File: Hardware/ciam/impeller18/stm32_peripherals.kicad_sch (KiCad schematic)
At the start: 31 parts, among them J21 TF-01, J22 USB_B_Micro, U73 W25Q128FVSIG, U74 USBLC6-2SC6

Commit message: added footprints
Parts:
- C108, C109, C110: footprint (none) -> Capacitor_SMD:C_0603_1608Metric
- D21, D22, D23, D24: footprint (none) -> user_lib:LED_RGB_promelec
- J22: footprint (none) -> user_lib:U-F-M5DD-W-2-SUS
- R259, R260, R261, R262, R263, R264, R265, R266, R267, R268, R269, R270, R271, R272, R273, R274, R275, R276, R277, R278: footprint (none) -> Resistor_SMD:R_0603_1608Metric
- U73: footprint (none) -> Package_SO:SOIC-8_5.23x5.23mm_P1.27mm
- U74: footprint (none) -> Package_TO_SOT_SMD:SOT-23-6
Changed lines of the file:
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@@
 			)
 		)
-		(property "Footprint" ""
+		(property "Footprint" "Resistor_SMD:R_0603_1608Metric"
 			(at 249.555 40.513 90)
 			(effects
@@
 			)
 		)
-		(property "Footprint" ""
+		(property "Footprint" "Resistor_SMD:R_0603_1608Metric"
 			(at 249.555 57.658 90)
 			(effects
@@
 			)
 		)
-		(property "Footprint" ""
+		(property "Footprint" "Resistor_SMD:R_0603_1608Metric"
 			(at 249.555 62.738 90)
 			(effects
@@
 			)
 		)
-		(property "Footprint" ""
+		(property "Footprint" "Resistor_SMD:R_0603_1608Metric"
 			(at 57.785 32.385 0)
 			(effects
@@
 			)
 		)
-		(property "Footprint" ""
+		(property "Footprint" "Resistor_SMD:R_0603_1608Metric"
 			(at 249.555 35.433 90)
 			(effects
@@
 			)
 		)
-		(property "Footprint" ""
+		(property "Footprint" "Resistor_SMD:R_0603_1608Metric"
 			(at 308.61 40.513 90)
 			(effects
@@
 			)
 		)
-		(property "Footprint" ""
+		(property "Footprint" "Resistor_SMD:R_0603_1608Metric"
 			(at 308.61 62.738 90)
 			(effects
@@
 			)
 		)
-		(property "Footprint" ""
+		(property "Footprint" "Package_SO:SOIC-8_5.23x5.23mm_P1.27mm"
 			(at 189.23 49.53 0)
 			(effects
@@
 			)
 		)
-		(property "Footprint" ""
+		(property "Footprint" "Resistor_SMD:R_0603_1608Metric"
 			(at 308.61 57.658 90)
 			(effects
@@
 			)
 		)
-		(property "Footprint" ""
+		(property "Footprint" "Resistor_SMD:R_0603_1608Metric"
 			(at 73.025 32.385 0)
 			(effects
@@
 			)
 		)
-		(property "Footprint" ""
+		(property "Footprint" "Capacitor_SMD:C_0603_1608Metric"
 			(at 30.48 114.935 0)
 			(effects
@@
 			)
 		)
-		(property "Footprint" ""
+		(property "Footprint" "Resistor_SMD:R_0603_1608Metric"
 			(at 120.015 119.38 0)
 			(effects
@@
 			)
 		)
-		(property "Footprint" ""
+		(property "Footprint" "Resistor_SMD:R_0603_1608Metric"
 			(at 50.165 32.385 0)
 			(effects
@@
 			)
 		)
-		(property "Footprint" ""
+		(property "Footprint" "Capacitor_SMD:C_0603_1608Metric"
 			(at 202.565 49.53 0)
 			(effects
@@
 			)
 		)
-		(property "Footprint" ""
+		(property "Footprint" "Package_TO_SOT_SMD:SOT-23-6"
 			(at 85.725 128.27 0)
 			(effects
@@
 			)
 		)
-		(property "Footprint" ""
+		(property "Footprint" "Resistor_SMD:R_0603_1608Metric"
 			(at 65.405 32.385 0)
 			(effects
@@
 			)
 		)
-		(property "Footprint" ""
+		(property "Footprint" "Resistor_SMD:R_0603_1608Metric"
 			(at 249.555 67.818 90)
 			(effects
@@
 			)
 		)
-		(property "Footprint" ""
+		(property "Footprint" "user_lib:U-F-M5DD-W-2-SUS"
 			(at 43.815 115.57 0)
 			(effects
@@
 			)
 		)
-		(property "Footprint" ""
+		(property "Footprint" "Resistor_SMD:R_0603_1608Metric"
 			(at 249.555 30.353 90)
 			(effects
@@
 			)
 		)
-		(property "Footprint" ""
+		(property "Footprint" "Resistor_SMD:R_0603_1608Metric"
 			(at 80.645 32.385 0)
 			(effects
@@
 			)
 		)
-		(property "Footprint" ""
+		(property "Footprint" "user_lib:LED_RGB_promelec"
 			(at 297.18 34.925 0)
 			(effects
@@
 			)
 		)
-		(property "Footprint" ""
+		(property "Footprint" "user_lib:LED_RGB_promelec"
 			(at 238.125 34.925 0)
 			(effects
@@
 			)
 		)
-		(property "Footprint" ""
+		(property "Footprint" "user_lib:LED_RGB_promelec"
 			(at 297.18 62.23 0)
 			(effects
@@
 			)
 		)
-		(property "Footprint" ""
+		(property "Footprint" "Resistor_SMD:R_0603_1608Metric"
 			(at 308.61 35.433 90)
 			(effects
@@
 			)
 		)
-		(property "Footprint" ""
+		(property "Footprint" "Resistor_SMD:R_0603_1608Metric"
 			(at 308.61 30.353 90)
 			(effects
@@
 			)
 		)
-		(property "Footprint" ""
+		(property "Footprint" "Resistor_SMD:R_0603_1608Metric"
 			(at 308.61 67.818 90)
 			(effects
@@
 			)
 		)
-		(property "Footprint" ""
+		(property "Footprint" "Resistor_SMD:R_0603_1608Metric"
 			(at 42.545 32.385 0)
 			(effects
@@
 			)
 		)
-		(property "Footprint" ""
+		(property "Footprint" "user_lib:LED_RGB_promelec"
 			(at 238.125 62.23 0)
 			(effects
@@
 			)
 		)
-		(property "Footprint" ""
+		(property "Footprint" "Capacitor_SMD:C_0603_1608Metric"
 			(at 97.79 28.575 0)
 			(effects
@@
 			)
 		)
-		(property "Footprint" ""
+		(property "Footprint" "Resistor_SMD:R_0603_1608Metric"
 			(at 120.015 109.22 0)
 			(effects

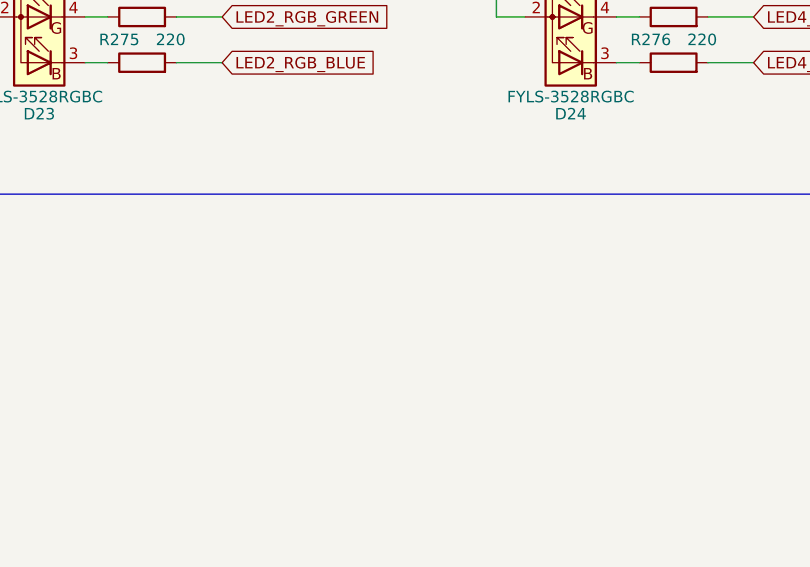
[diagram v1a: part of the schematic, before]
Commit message: Minor changes
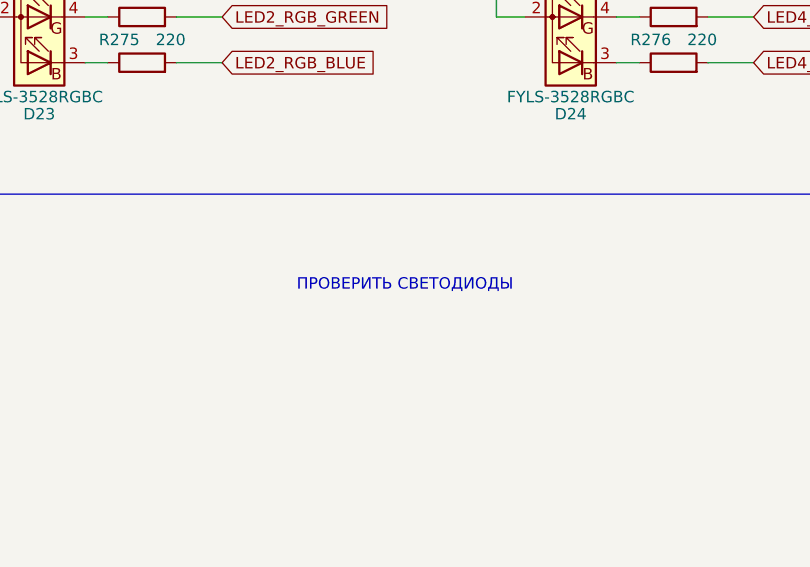
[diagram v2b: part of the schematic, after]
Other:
- note added: "ПРОВЕРИТЬ СВЕТОДИОДЫ"
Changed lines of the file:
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@@
+		)
+	)
+	(text "ПРОВЕРИТЬ СВЕТОДИОДЫ"
+		(exclude_from_sim no)
+		(at 278.765 90.805 0)
+		(effects
+			(font
+				(size 1.27 1.27)
+			)
 		)
 	)

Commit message: Updated packeges
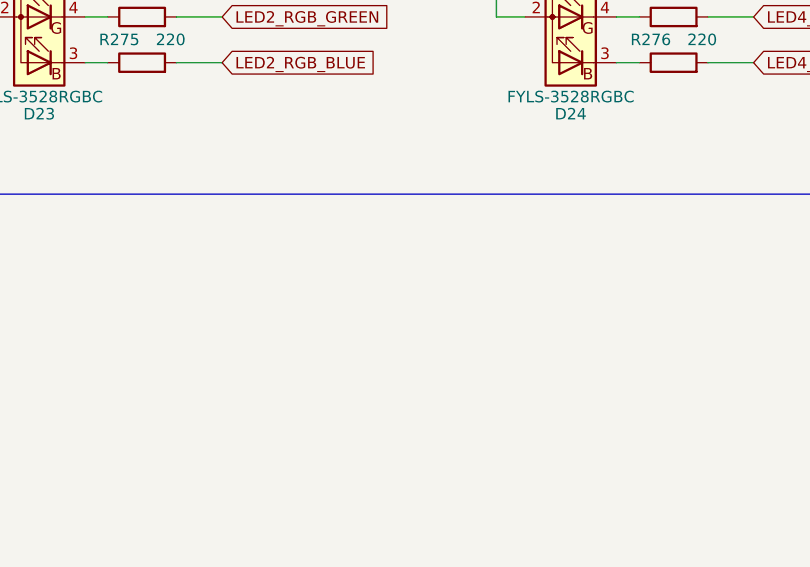
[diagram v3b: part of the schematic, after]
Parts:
- U73: footprint Package_SO:SOIC-8_5.23x5.23mm_P1.27mm -> user_lib:SOIC-8_5.23x5.23mm_P1.27mm
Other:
- note removed: "ПРОВЕРИТЬ СВЕТОДИОДЫ"
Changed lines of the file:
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@@
-		)
-	)
-	(text "ПРОВЕРИТЬ СВЕТОДИОДЫ"
-		(exclude_from_sim no)
-		(at 278.765 90.805 0)
-		(effects
-			(font
-				(size 1.27 1.27)
-			)
 		)
 	)
@@
 			)
 		)
-		(property "Footprint" "Package_SO:SOIC-8_5.23x5.23mm_P1.27mm"
+		(property "Footprint" "user_lib:SOIC-8_5.23x5.23mm_P1.27mm"
 			(at 189.23 49.53 0)
 			(effects

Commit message: Updated packeges
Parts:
- J21: footprint (none) -> sd:TF01A-NEW
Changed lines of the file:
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@@
 			)
 		)
-		(property "Footprint" ""
+		(property "Footprint" "sd:TF01A-NEW"
 			(at 170.18 33.655 0)
 			(effects
